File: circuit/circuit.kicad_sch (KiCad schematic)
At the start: 36 parts, among them IC1 BNO085, J1 Conn_01x04_Pin, J3 USB_C_Receptacle_USB2.0, J4 Conn_01x10_Pin, Q1 IRLML6244, U1 ESP32-C3-WROOM-02, U2 BD33FC0FP

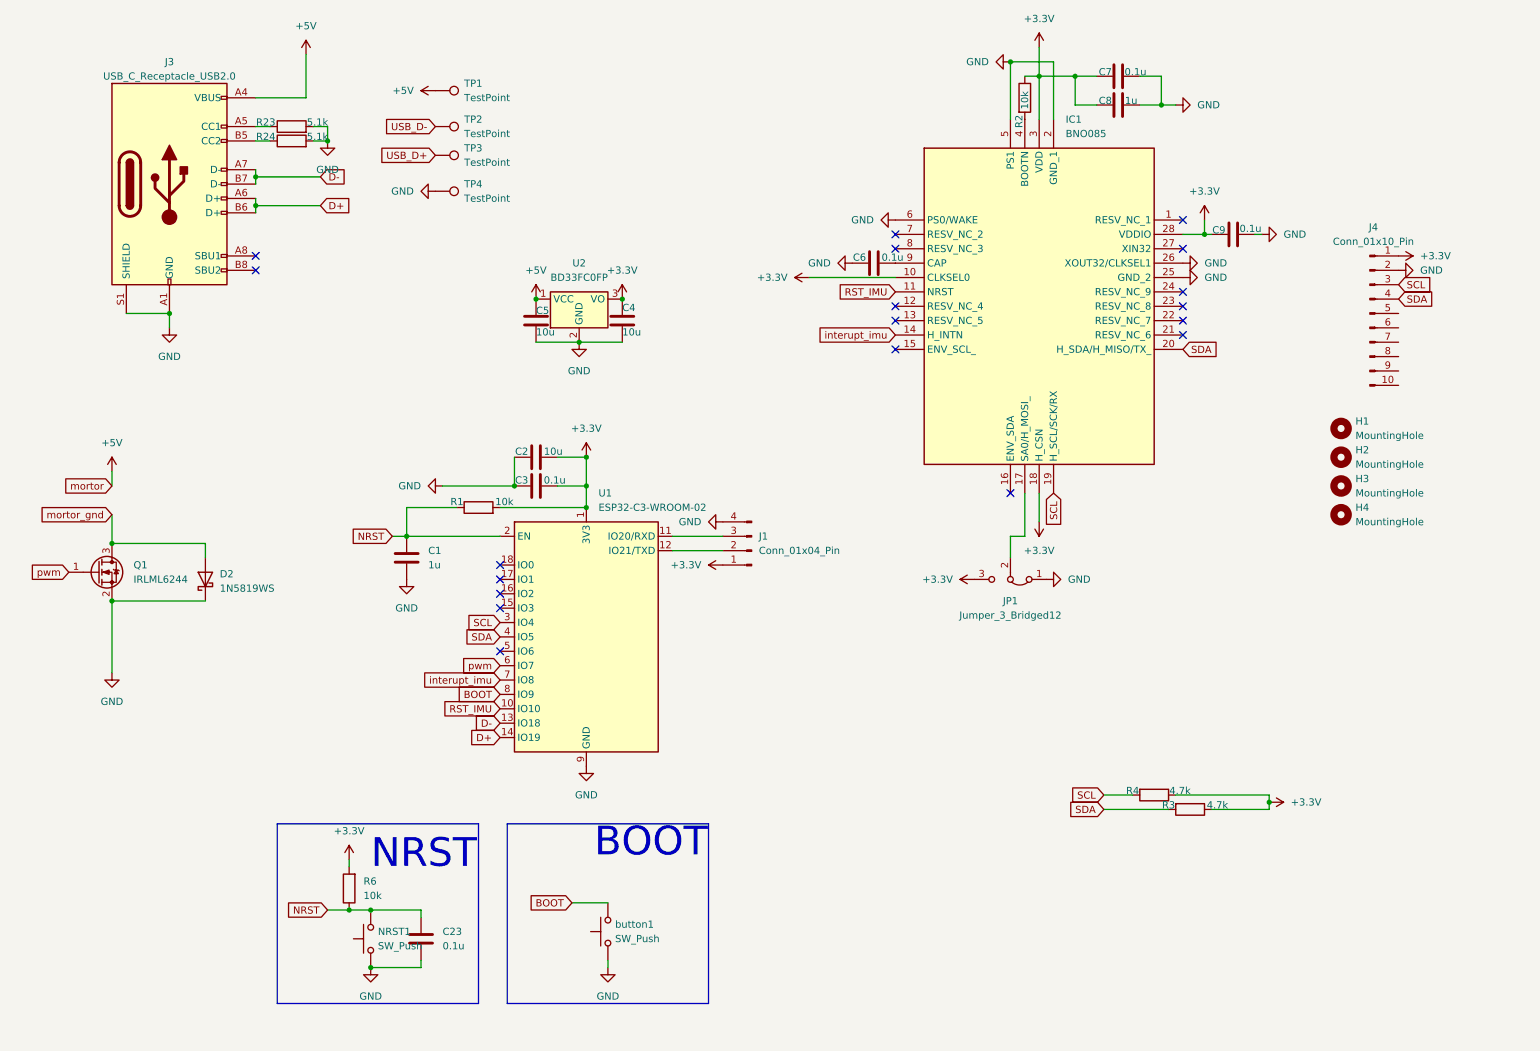
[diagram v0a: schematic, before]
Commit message: 基板動いた．pio最終版
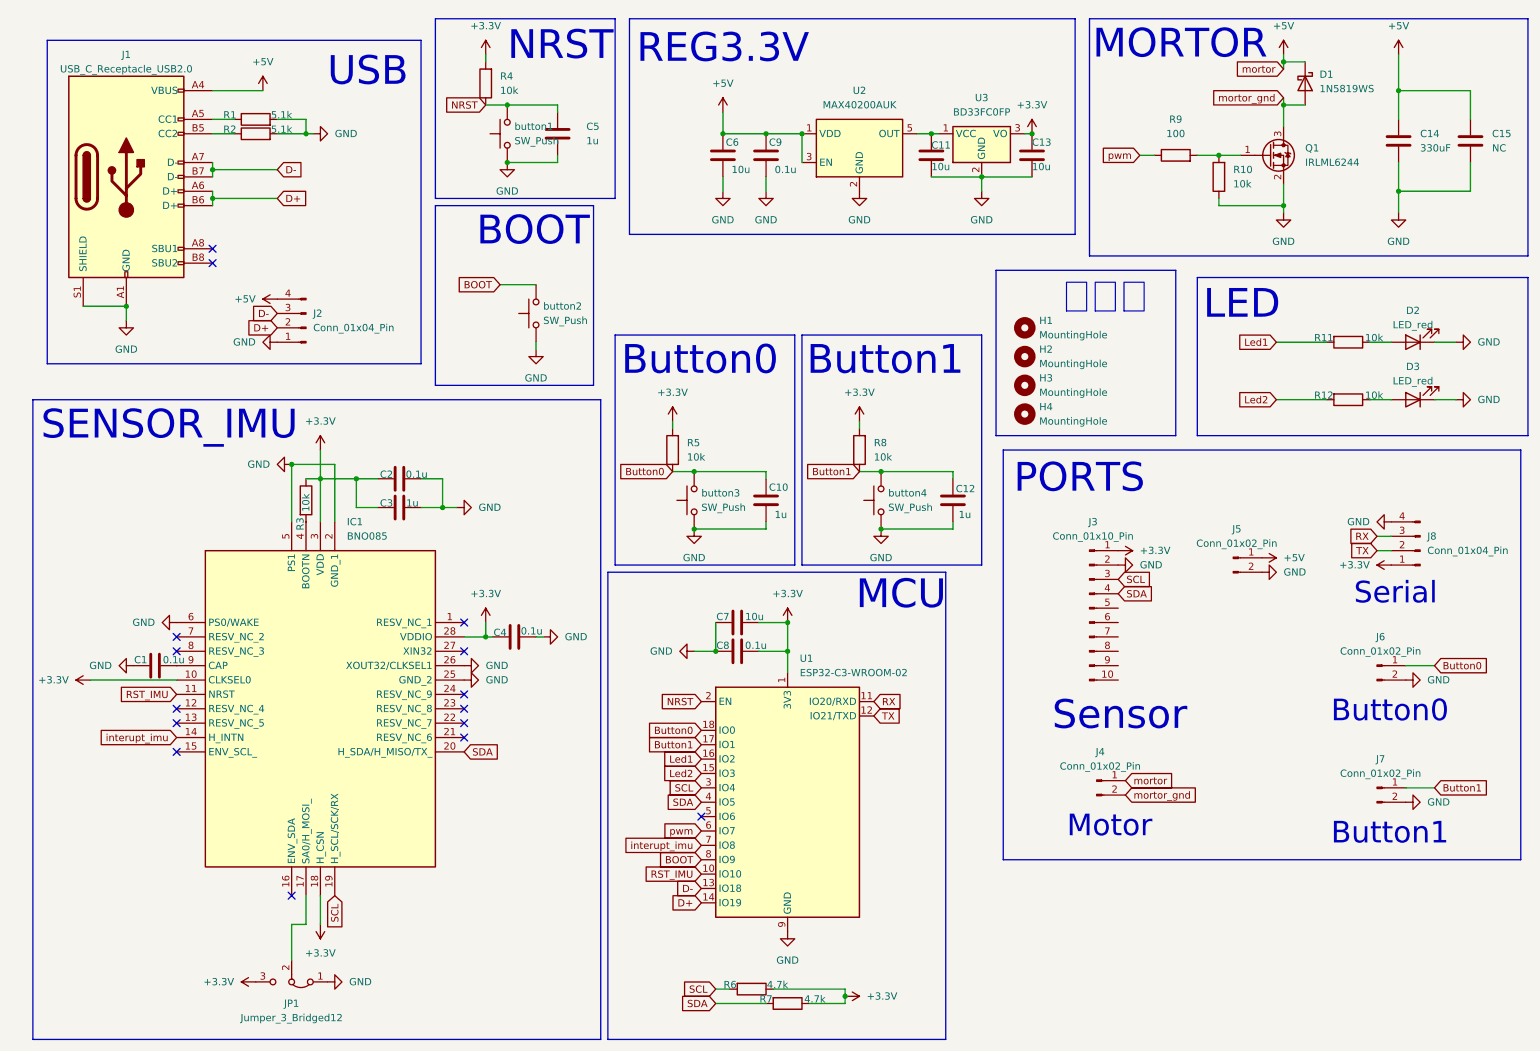
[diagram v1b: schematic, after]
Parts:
- removed C1: 1u, Capacitor_SMD:C_0603_1608Metric, symbol Device:C
- removed R1: 10k, Resistor_SMD:R_0603_1608Metric_Pad0.98x0.95mm_HandSolder, symbol Device:R
- removed TP1, TP2, TP3, TP4: TestPoint, TestPoint:TestPoint_Pad_D1.5mm, symbol Connector:TestPoint
- added C10, C12: 1u, Capacitor_SMD:C_0603_1608Metric, symbol Device:C
- added C14: 330uF, Capacitor_SMD:C_Elec_10x10.2, symbol Device:C
- added C15: NC, Capacitor_THT:C_Radial_D5.0mm_H7.0mm_P2.00mm, symbol Device:C
- added C6: 10u, Capacitor_SMD:C_0603_1608Metric, symbol Device:C
- added C9: 0.1u, Capacitor_SMD:C_0603_1608Metric, symbol Device:C
- added D2, D3: LED_red, LED_SMD:LED_0603_1608Metric_Pad1.05x0.95mm_HandSolder, symbol Device:LED
- added J2: Conn_01x04_Pin, Connector_PinSocket_2.54mm:PinSocket_1x04_P2.54mm_Vertical, symbol Connector:Conn_01x04_Pin
- added J4, J6, J7: Conn_01x02_Pin, Connector_PinHeader_2.54mm:PinHeader_1x02_P2.54mm_Vertical, symbol Connector:Conn_01x02_Pin
- added J5: Conn_01x02_Pin, Connector_JST:JST_XH_B2B-XH-A_1x02_P2.50mm_Vertical, symbol Connector:Conn_01x02_Pin
- added R10, R11, R12, R5, R8: 10k, Resistor_SMD:R_0603_1608Metric_Pad0.98x0.95mm_HandSolder, symbol Device:R
- added R9: 100, Resistor_SMD:R_0603_1608Metric_Pad0.98x0.95mm_HandSolder, symbol Device:R
- added U2: MAX40200AUK, Package_TO_SOT_SMD:SOT-23-5, symbol Analog_Switch:MAX40200AUK
- added button3, button4: SW_Push, Button_Switch_SMD:SW_SPST_PTS810, symbol Switch:SW_Push
- C5: renamed from C23; value 0.1u -> 1u
- renumbered C6 to C1, C5 to C11, C4 to C13, C7 to C2, C8 to C3, C9 to C4, C2 to C7, C3 to C8, D2 to D1, J3 to J1, J4 to J3, J1 to J8, R23 to R1, R24 to R2, R2 to R3, R6 to R4, R4 to R6, R3 to R7, U2 to U3, NRST1 to button1, button1 to button2
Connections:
- net +3.3V: now also R5.2, R8.2
- net +5V: now also D1.1 (K), C14.1, C15.1, C6.1, C9.1, J2.4 (Pin_4), J4.1 (Pin_1), J5.1 (Pin_1), U2.1 (VDD), U2.3 (EN); no longer C11.1, U3.1 (VCC)
- net D+: now also J2.2 (Pin_2)
- net D-: now also J2.3 (Pin_3)
- net GND: now also C10.2, C12.2, C14.2, C15.2, C6.2, C9.2, D2.1 (K), D3.1 (K), J2.1 (Pin_1), J5.2 (Pin_2), J6.2 (Pin_2), J7.2 (Pin_2), R10.1, U2.2 (GND), button3.1, button4.1; no longer D1.1 (K)
- net mortor_gnd: now also J4.2 (Pin_2)
- net pwm: now also R9.1; no longer Q1.1 (G)
- net TX: now reaches J8.2 (Pin_2), U1.12 (IO21/TXD)
- net RX: now reaches J8.3 (Pin_3), U1.11 (IO20/RXD)
- net Led2: now reaches U1.15 (IO3)
- net Led2: now also R12.2
- net Led1: now reaches U1.16 (IO2)
- net Led1: now also R11.2
- net Button1: now reaches U1.17 (IO1)
- net Button1: now also C12.1, J7.1 (Pin_1), R8.1, button4.2
- net Button0: now reaches U1.18 (IO0)
- net Button0: now also C10.1, J6.1 (Pin_1), R5.1, button3.2
- new net: C11.1, U2.5 (OUT), U3.1 (VCC)
- new net: D2.2 (A), R11.1
- new net: Q1.1 (G), R10.2, R9.2
- new net: D3.2 (A), R12.1
- no-connect marks 19 -> 15
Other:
- note added: "Button0"
- note added: "Button1"
- note added: "LED"
- note added: "MCU"
- note added: "MORTOR"
- note added: "Motor"
- note added: "PORTS"
- note added: "REG3.3V"
- note added: "SENSOR_IMU"
- note added: "Sensor"
- note added: "Serial"
- note added: "USB"
- note added: "取付穴"
- moved on the sheet: C1, C11, C13, C2, C3, C4, C5, C7, C8, D1, H1, H2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
